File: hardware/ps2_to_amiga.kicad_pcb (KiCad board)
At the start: 2 copper layers, 22.9 x 15.2 mm, 7 parts, among them J1 Conn_01x05, J2 Conn_01x04, J3 Conn_02x03_Odd_Even, J4 DIN-5_180degree, U1 ATtiny85-20S

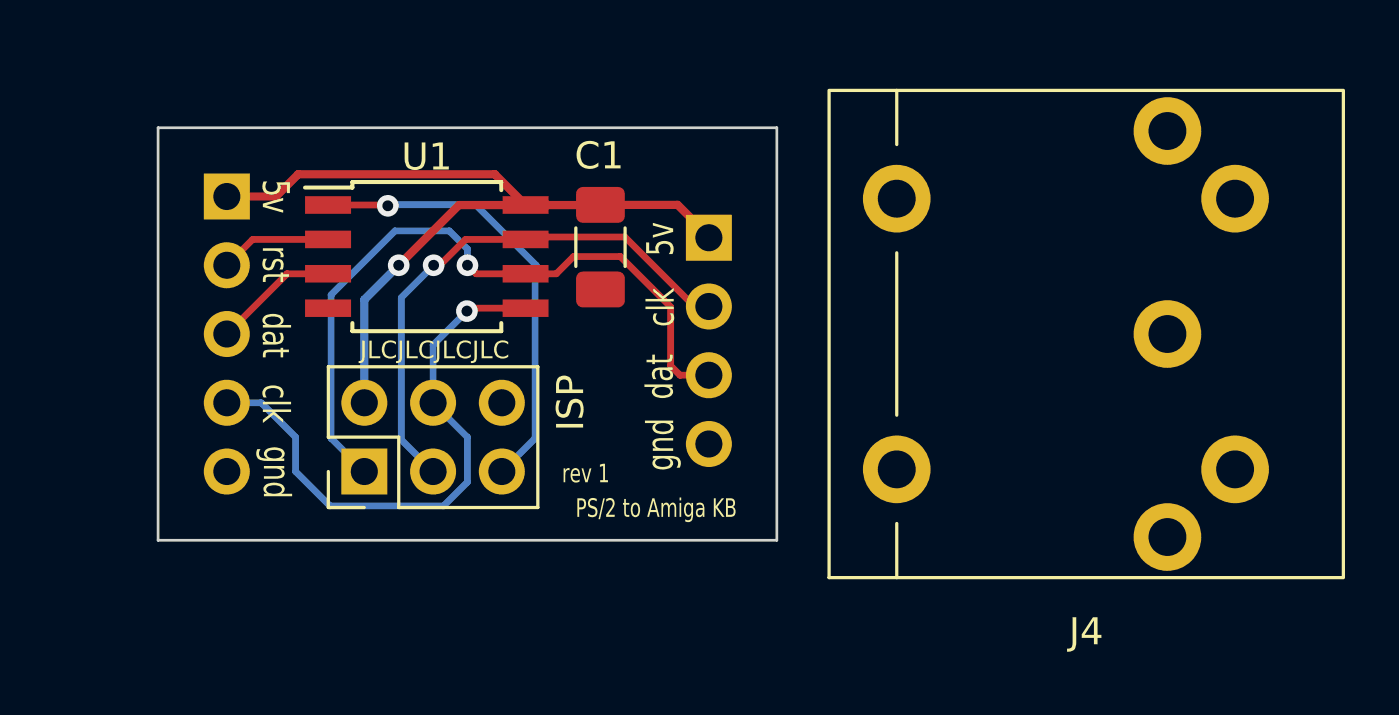
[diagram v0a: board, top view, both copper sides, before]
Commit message: Design rev2 pcb
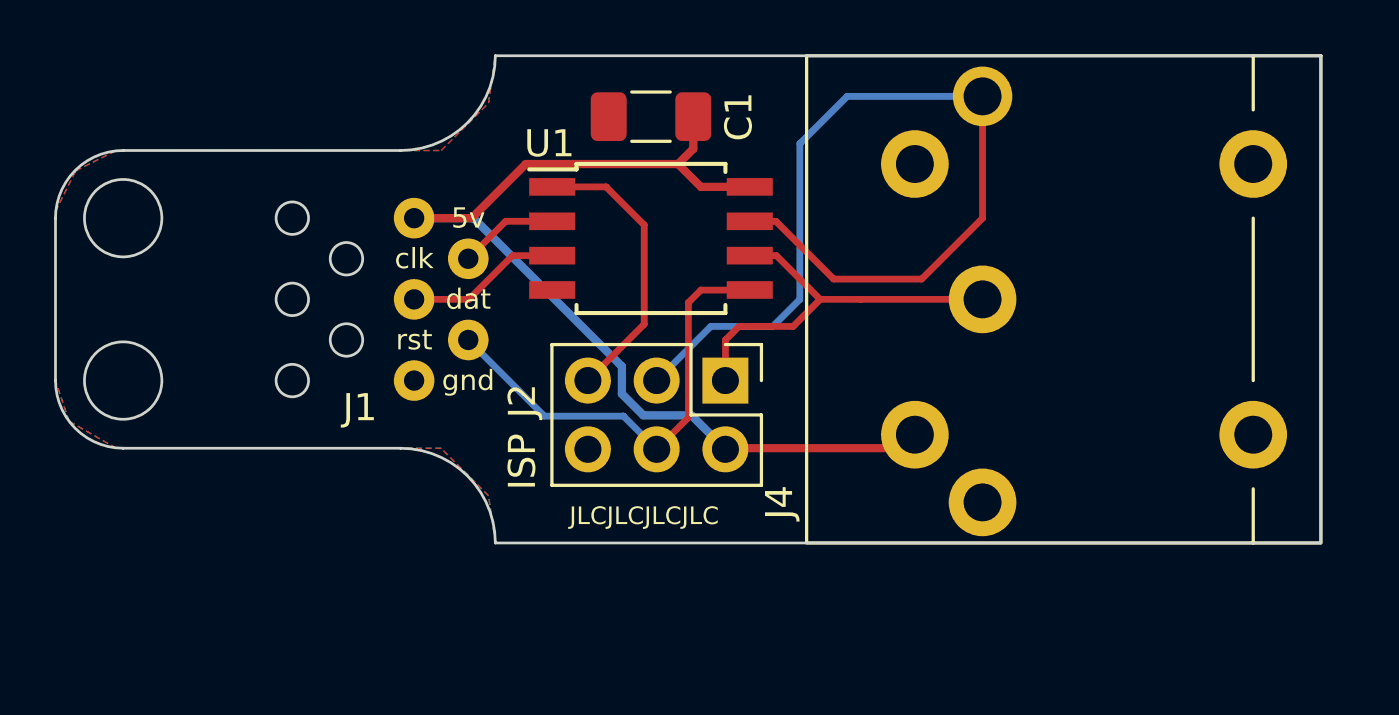
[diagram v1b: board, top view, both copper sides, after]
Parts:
- removed J3: Conn_02x03_Odd_Even, Connector_PinHeader_2.54mm:PinHeader_2x03_P2.54mm_Vertical
- J1: footprint Connector_PinHeader_2.54mm:PinHeader_1x05_P2.54mm_Vertical -> Library:AMIGA_KB_PADS
- J2: value Conn_01x04 -> AVR-ISP-6; footprint Connector_PinHeader_2.54mm:PinHeader_1x04_P2.54mm_Vertical -> Connector_PinHeader_2.54mm:PinHeader_2x03_P2.54mm_Vertical
- moved J1 8.56 mm to (139.8, 80.0), turned to -90 degrees
- moved U1 8.31 mm to (147.8, 77.8)
- moved REF** 5.47 mm to (148.5, 75.2)
- moved J2 5.31 mm to (150.5, 83.0), turned to -90 degrees
- moved C1 5.17 mm to (147.8, 73.2), turned to 180 degrees
- moved J4 1.53 mm to (163.0, 80.0), turned to 180 degrees
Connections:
- J1 pad 2: AMIGA_RST -> AMIGA_CLK
- J1 pad 4: AMIGA_CLK -> AMIGA_RST
- J2 pad 1: +5V -> PS2_DAT
- J2 pad 2: PS2_CLK -> +5V
- J2 pad 3: PS2_DAT -> PS2_CLK
- J2 pad 4: GND -> AMIGA_RST
- J4 pad 1: unconnected-(J4-Pad1) -> PS2_CLK
- J4 pad 2: unconnected-(J4-Pad2) -> PS2_DAT
- J4 pad 4: unconnected-(J4-Pad4) -> GND
- J4 pad 5: unconnected-(J4-Pad5) -> +5V
- J4 pad 6: (no net) -> GND
- U1 pad 2: AMIGA_RST -> AMIGA_CLK
- U1 pad 5: AMIGA_CLK -> AMIGA_RST
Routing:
- net AMIGA_CLK: track 21.2 -> 3.67 mm, vias 1 -> 0
- net PS2_CLK: track 20.3 -> 34.1 mm, vias 1 -> 0
- net AMIGA_RST: track 4.14 -> 17.0 mm
- net PS2_DAT: track 26.3 -> 14.3 mm, vias 1 -> 0
- net +5V: track 30.4 -> 38.9 mm, vias 1 -> 0
- net /ISP_RST: track 16.8 -> 10.6 mm, vias 1 -> 0
- net AMIGA_DAT: track 4.66 -> 5.77 mm
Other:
- board size 22.9 x 15.2 mm -> 46.8 x 18 mm
- board text added: "rev 2"
- board text removed: "rev 1"
